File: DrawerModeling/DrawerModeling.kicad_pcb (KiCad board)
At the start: 2 copper layers, 167 x 119.6 mm, 100 parts, among them J1 Conn_01x05_Pin, Q1 2N3904, Q2 2N3904, Q3 2N3906, Q4 2N3904, Q5 2N3904, U10 TL072, U11 TLP222A, U12 TLP222A, U13 TL072, U14 LM13700, U15 TL072, U16 TLP222A, U17 TLP222A, U18 MCP4725xxx-xCH, U19 XC6206PxxxMR, U2 TL072, U6 TL072, U7 STM32F411CCUx, U8 LT1011, U9 TL072, Y1 Crystal

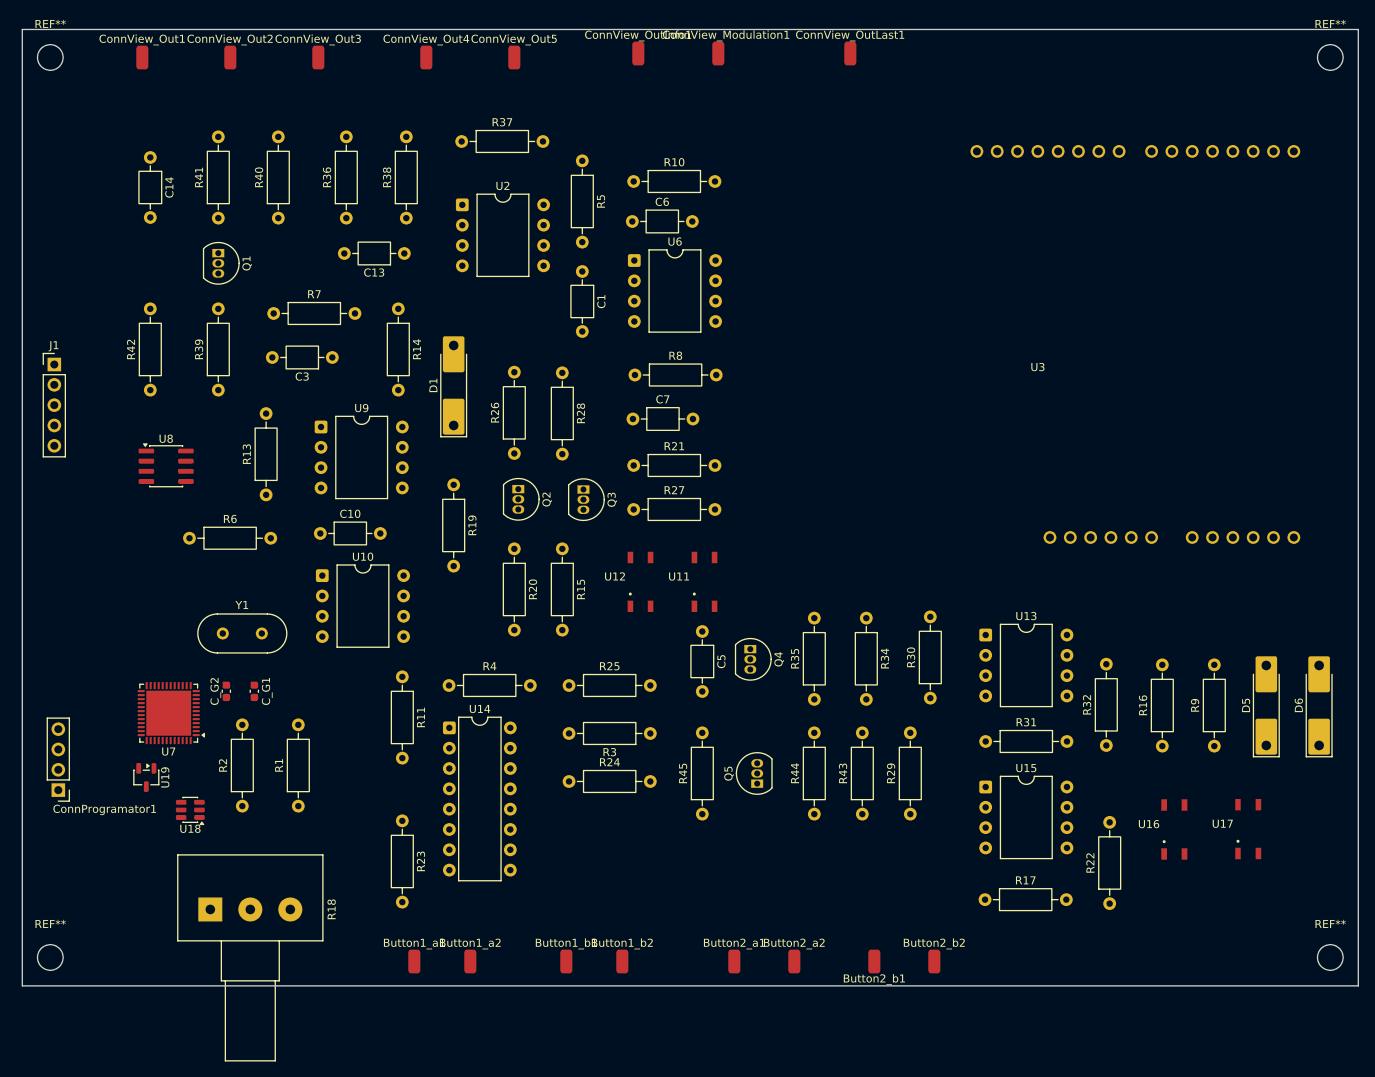
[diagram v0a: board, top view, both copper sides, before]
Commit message: recovery after bad days
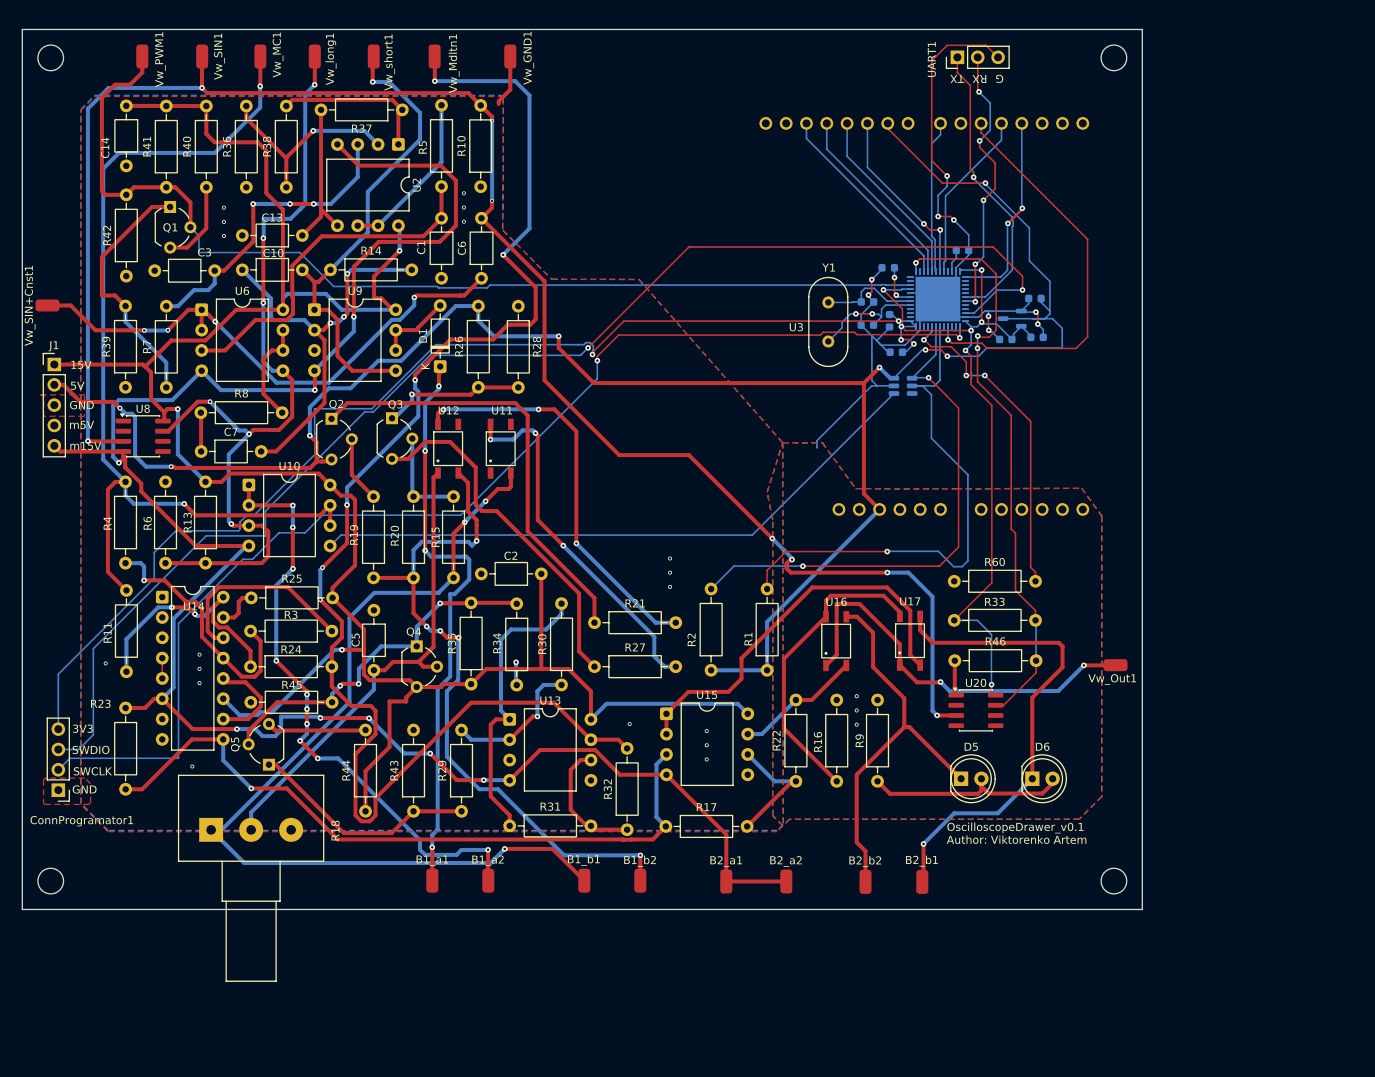
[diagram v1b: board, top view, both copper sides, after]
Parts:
- removed the REF** at (25.0, 140.5)
- removed the REF** at (25.0, 28.0)
- removed the REF** at (185.0, 140.5)
- removed the REF** at (185.0, 28.0)
- added C2: C, Capacitor_THT:C_Axial_L3.8mm_D2.6mm_P7.50mm_Horizontal, F.Cu at (86.4, 92.5)
- added C_s1: 100n, Capacitor_SMD:C_0603_1608Metric, B.Cu at (130.7, 64.8)
- added C_s3: 100n, Capacitor_SMD:C_0603_1608Metric, B.Cu at (144.4, 63.2)
- added C_s4: 100n, Capacitor_SMD:C_0603_1608Metric, B.Cu at (129.9, 60.9)
- added C_s5: 1u, Capacitor_SMD:C_0603_1608Metric, B.Cu at (148.1, 58.1)
- added C_s6: 1u, Capacitor_SMD:C_0603_1608Metric, B.Cu at (148.3, 63.0)
- added C_s7: C, Capacitor_SMD:C_0603_1608Metric, B.Cu at (139.0, 52.1)
- added C_s8: 100n, Capacitor_SMD:C_0603_1608Metric, B.Cu at (129.7, 54.3)
- added R33: R, Resistor_THT:R_Axial_DIN0207_L6.3mm_D2.5mm_P10.16mm_Horizontal, F.Cu at (148.2, 98.4)
- added R46: R, Resistor_THT:R_Axial_DIN0207_L6.3mm_D2.5mm_P10.16mm_Horizontal, F.Cu at (138.1, 103.4)
- added R60: 10k, Resistor_THT:R_Axial_DIN0207_L6.3mm_D2.5mm_P10.16mm_Horizontal, F.Cu at (138.0, 93.5)
- added REF**: MountingHole_3.2mm_M3, MountingHole:MountingHole_3.2mm_M3, F.Cu at (25.1, 130.9)
- added REF**: MountingHole_3.2mm_M3, MountingHole:MountingHole_3.2mm_M3, F.Cu at (157.9, 130.9)
- added REF**: MountingHole_3.2mm_M3, MountingHole:MountingHole_3.2mm_M3, F.Cu at (25.1, 28.1)
- added REF**: MountingHole_3.2mm_M3, MountingHole:MountingHole_3.2mm_M3, F.Cu at (157.9, 28.1)
- added U20: LT1011, Package_SO:SOIC-8_3.9x4.9mm_P1.27mm, F.Cu at (140.7, 109.6)
- added UART1: Conn_01x03_Pin, Connector_PinHeader_2.54mm:PinHeader_1x03_P2.54mm_Vertical, F.Cu at (138.4, 28.0)
- added Vw_GND1: Conn_01x01, Connector_Wire:SolderWirePad_1x01_SMD_1.5x3mm, F.Cu at (82.5, 27.9)
- C_G1, C_G2, U18, U19: moved to B.Cu
- D1: value D -> 1N4148; footprint Diode_SMD:D_MELF-RM10_Universal_Handsoldering -> Diode_THT:D_DO-35_SOD27_P7.62mm_Horizontal
- D5, D6: value D -> LED; footprint Diode_SMD:D_MELF-RM10_Universal_Handsoldering -> LED_THT:LED_D5.0mm
- Q1, Q2, Q3, Q4, Q5: footprint Package_TO_SOT_THT:TO-92_Inline -> Package_TO_SOT_THT:TO-92_Wide
- U7: value STM32F411CCUx -> STM32F401CCUx; moved to B.Cu
- moved U19 122.5 mm to (145.2, 60.6), turned to 180 degrees
- moved U7 109.2 mm to (135.9, 58.2), turned to 0 degrees
- moved U18 103.7 mm to (131.6, 69.0), turned to 0 degrees
- moved C_G2 93.8 mm to (127.2, 58.6), turned to 180 degrees
- moved C_G1 89.3 mm to (127.1, 61.5), turned to 0 degrees
- moved Y1 86.3 mm to (122.2, 58.6), turned to -90 degrees
- moved Vw_Out1 83.3 mm to (158.2, 104.0), turned to -90 degrees
- moved Q5 61.1 mm to (52.3, 116.4)
- moved R1 61.0 mm to (114.6, 104.6)
- moved R2 61.0 mm to (107.6, 104.6)
- moved R32 60.8 mm to (97.1, 124.5)
- moved R31 60.4 mm to (82.4, 124.0)
- moved U13 60.4 mm to (82.4, 110.7)
- moved R29 56.1 mm to (76.4, 122.2)
- moved R43 56.1 mm to (70.4, 122.2)
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- renumbered Button1_a1 to B1_a1, Button1_a2 to B1_a2, Button1_b1 to B1_b1, Button1_b2 to B1_b2, Button2_a1 to B2_a1, Button2_a2 to B2_a2, Button2_b1 to B2_b1, Button2_b2 to B2_b2, ConnView_OutInfo1 to Vw_MC1, ConnView_Modulation1 to Vw_Mdltn1, ConnView_OutLast1 to Vw_Out1, ConnView_Out1 to Vw_PWM1, ConnView_Out2 to Vw_SIN+Cnst1, ConnView_Out3 to Vw_SIN1, ConnView_Out5 to Vw_long1, ConnView_Out4 to Vw_short1
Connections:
- Q1 pad 2: Net-(ConnView_Out1-Pin_1) -> /PWM
- R41 pad 1: Net-(ConnView_Out1-Pin_1) -> /PWM
- R42 pad 2: Net-(ConnView_Out1-Pin_1) -> /PWM
- U7 pad 10: unconnected-(U7-PA0-Pad10) -> /PWM
- U7 pad 13: unconnected-(U7-PA3-Pad13) -> Net-(U7-PA3)
- U7 pad 22: unconnected-(U7-VCAP1-Pad22) -> Net-(U7-VCAP1)
- U7 pad 30: unconnected-(U7-PA9-Pad30) -> /TX
- U7 pad 31: unconnected-(U7-PA10-Pad31) -> /RX
- U7 pad 44: unconnected-(U7-BOOT0-Pad44) -> Net-(U7-BOOT0)
- U7 pad 7: unconnected-(U7-NRST-Pad7) -> Net-(U7-NRST)
- U7 pad 8: unconnected-(U7-VSSA-Pad8) -> GND
- Vw_PWM1 pad 1: Net-(ConnView_Out1-Pin_1) -> /PWM
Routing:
- net /V15: track 0.00 -> 278.5 mm, vias 0 -> 3
- net /V5: track 0.00 -> 257.9 mm, vias 0 -> 8
- net /V15m: track 0.00 -> 248.2 mm, vias 0 -> 8
- net /3V3: track 0.00 -> 241.5 mm, vias 0 -> 11
- net Net-(U20--): track 0.00 -> 218.7 mm, vias 0 -> 8
- net Net-(Vw_Mdltn1-Pin_1): track 0.00 -> 175.3 mm, vias 0 -> 6
- net /SWDIO: track 0.00 -> 166.3 mm, vias 0 -> 2
- net /SWCLK: track 0.00 -> 148.6 mm, vias 0 -> 2
- net GND: track 0.00 -> 132.6 mm, vias 0 -> 31
- net /PWM: track 0.00 -> 130.1 mm
- net Net-(B1_b1-Pin_1): track 0.00 -> 117.1 mm, vias 0 -> 3
- net Net-(U10B--): track 0.00 -> 116.9 mm, vias 0 -> 2
- net Net-(U10A-+): track 0.00 -> 105.7 mm, vias 0 -> 6
- net Net-(U15A-+): track 0.00 -> 87.5 mm, vias 0 -> 1
- net Net-(B1_b2-Pin_1): track 0.00 -> 85.9 mm, vias 0 -> 5
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- added copper zone on B.Cu, net GND
- added copper zone on F.Cu, net GND
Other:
- board size 167 x 119.6 mm -> 140 x 110 mm
- board text added: "15V"
- board text added: "3V3"
- board text added: "5V"
- board text added: "G"
- board text added: "GND"
- board text added: "OscilloscopeDrawer_v0.1 Author: Viktorenko Artem"
- board text added: "RX"
- board text added: "SWCLK"
- board text added: "SWDIO"
- board text added: "TX"
- board text added: "m15V"
- board text added: "m5V"
